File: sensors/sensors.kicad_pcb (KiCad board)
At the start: 2 copper layers, 73 x 56 mm, 73 parts, among them J1 GPIO, J3 JP_PWM, J4 JP_ADC, J5 JP_GPS, J6 JP_RADIO, J7 JP_RCIN, SW1 SW_SPDT_321, SW2 SW_SPDT_321, U1 SC16IS752IPW, U2 PCA9685PW, U3 ICM-42605, U4 IST8310, U5 MS5611-01BA, U6 74LVC1G86, U7 ADS1115IDGS, Y1 14.7456MHz, Y2 ASE-xxxMHz

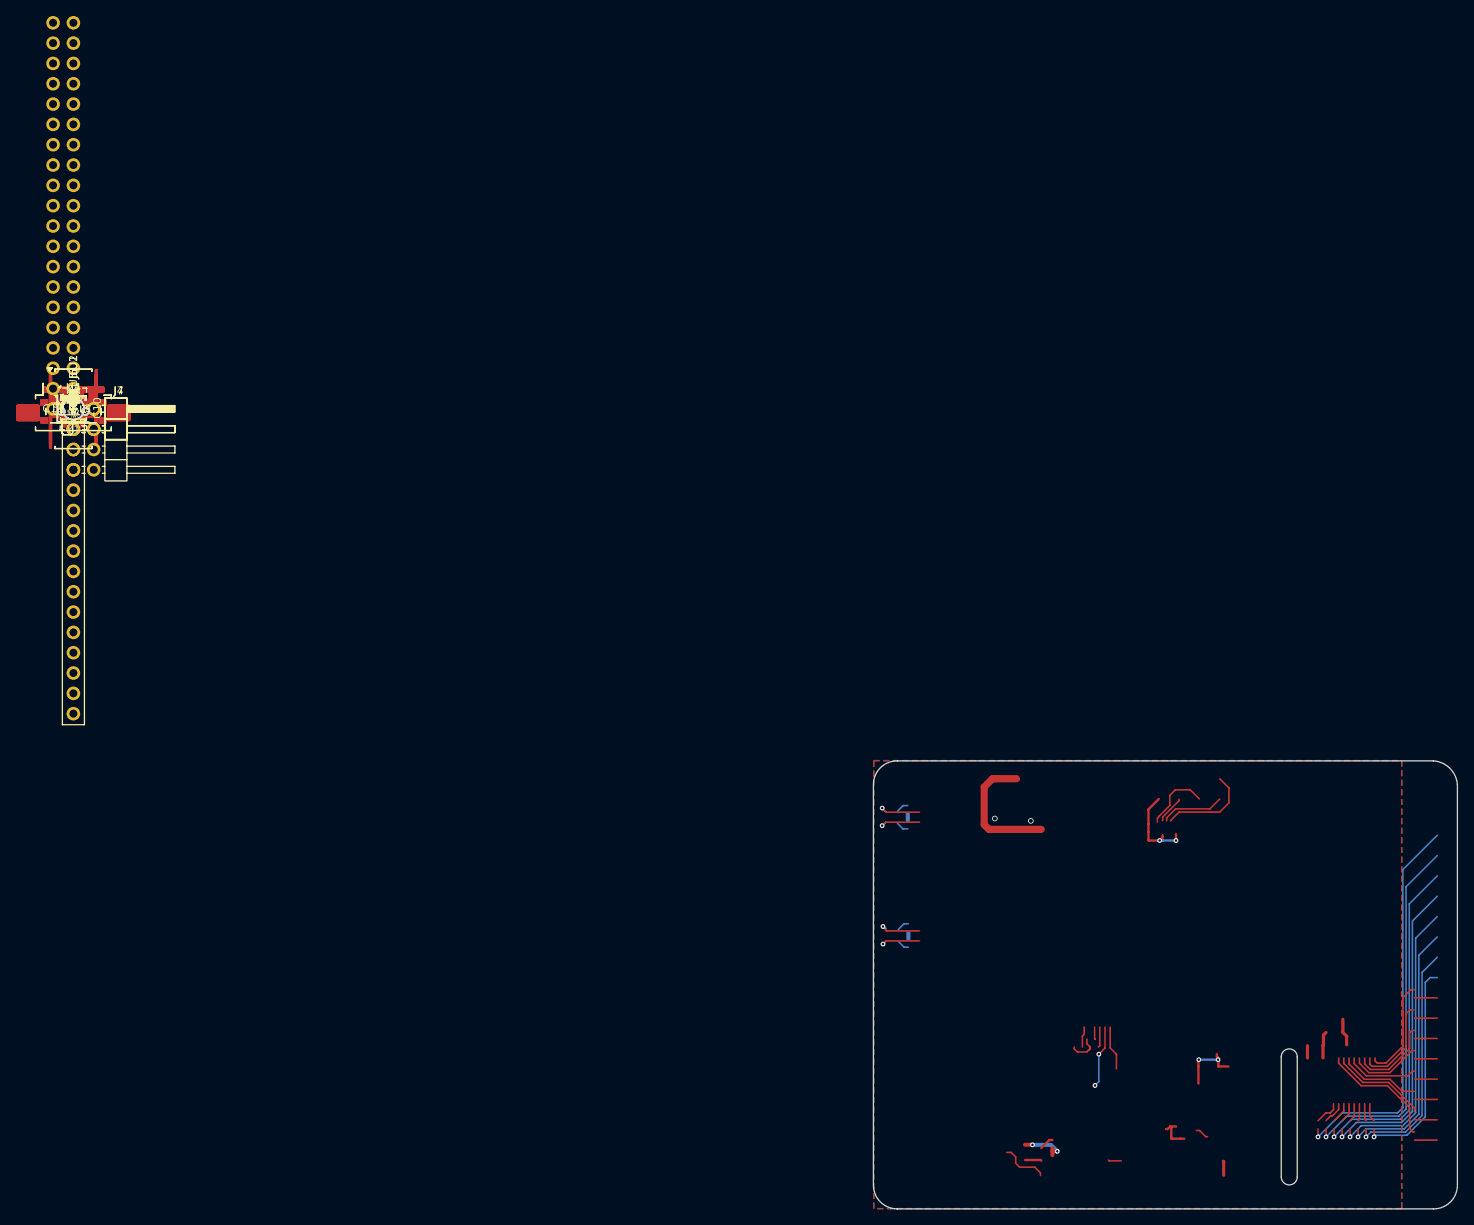
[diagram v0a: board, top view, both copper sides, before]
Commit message: routing
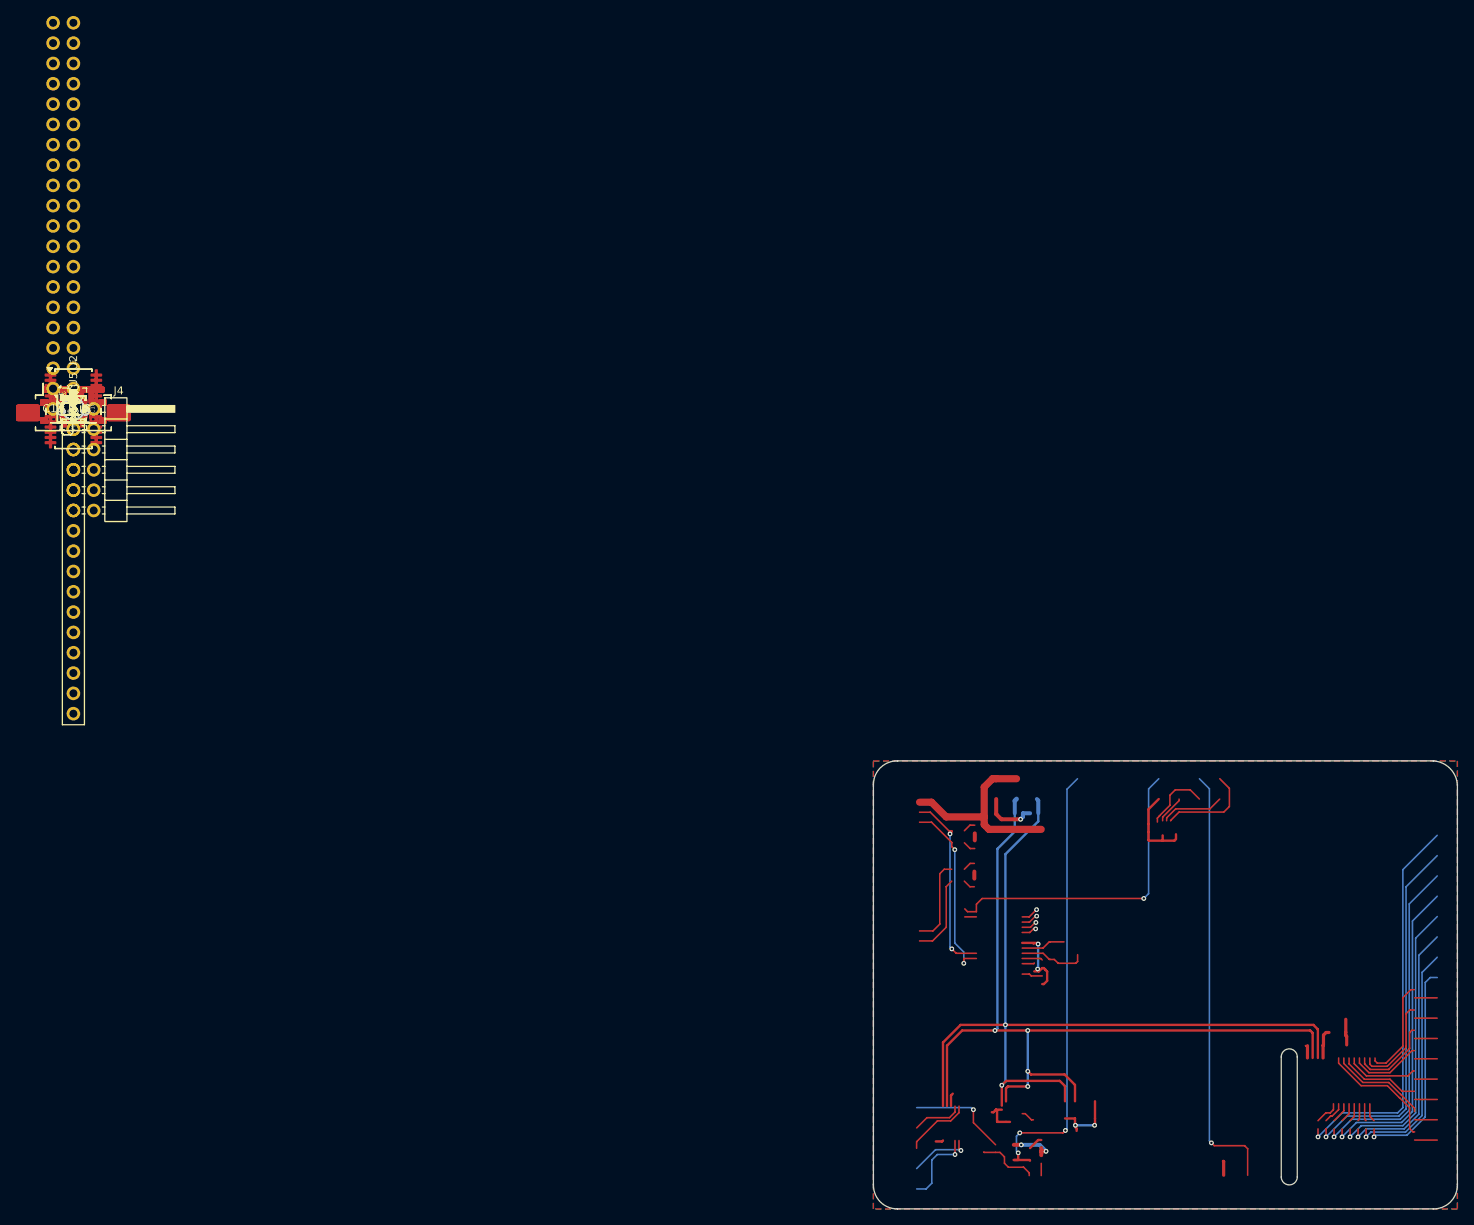
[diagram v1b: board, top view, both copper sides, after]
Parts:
- removed J7: JP_RCIN, Connector_PinHeader_2.54mm:PinHeader_2x02_P2.54mm_Horizontal
- D1: value RXA_GREEN -> TXA_RED; moved to F.Cu
- D2: value TXA_RED -> RXA_GREEN; moved to F.Cu
- D3: value RXB_GREEN -> TXB_RED; moved to F.Cu
- D4: value TXB_RED -> RXB_GREEN; moved to F.Cu
- J4: footprint Connector_PinHeader_2.54mm:PinHeader_2x04_P2.54mm_Horizontal -> Connector_PinHeader_2.54mm:PinHeader_2x06_P2.54mm_Horizontal
- R11, R6, R8, R9: moved to F.Cu
- R33, R34: moved to B.Cu
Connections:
- D1 pad 1: /UART/RXA -> /UART/TXA
- D2 pad 1: /UART/TXA -> /UART/RXA
- D3 pad 1: /UART/RXB -> /UART/TXB
- D4 pad 1: /UART/TXB -> /UART/RXB
- J4 pad 1: GND -> /ADC/AIN0
- J4 pad 3: GND -> /ADC/AIN1
- J4 pad 5: /ADC/AIN3 -> /ADC/AIN2
- J4 pad 6: /ADC/AIN2 -> GND
- J4 pad 7: /ADC/AIN1 -> /ADC/AIN3
- J4 pad 8: /ADC/AIN0 -> GND
- R10 pad 2: /UART/TXB -> /UART/RXB
- R7 pad 2: /UART/TXA -> /UART/RXA
- U6 pad 1: /RC inverter/RC -> /RCIN
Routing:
- net /GPIO3/SCL1: track 0.00 -> 110.1 mm, vias 0 -> 2
- net /GPIO2/SDA1: track 0.00 -> 107.7 mm, vias 0 -> 4
- net /GPIO15/RXD0: track 2.07 -> 56.7 mm, vias 0 -> 3
- net /GPIO25: track 0.00 -> 54.3 mm, vias 0 -> 1
- net /SDIODAT0/GPIO24: track 0.00 -> 39.5 mm, vias 0 -> 1
- net /UART/TXB: track 5.42 -> 23.2 mm, vias 1 -> 2
- net /UART/RXB: track 5.30 -> 23.0 mm, vias 1 -> 2
- net +3V3: track 39.4 -> 53.0 mm, vias 6 -> 7
- net /RCIN: track 0.00 -> 12.7 mm, vias 0 -> 1
- net /ADC/AIN0: track 0.00 -> 10.0 mm, vias 0 -> 1
- net +5V: track 18.1 -> 27.2 mm
- net /ADC/AIN2: track 0.00 -> 8.45 mm
- net /ADC/AIN1: track 0.00 -> 7.91 mm, vias 0 -> 1
- net /ADC/AIN3: track 0.00 -> 6.37 mm
- net /UART/TXA: track 5.40 -> 10.9 mm, vias 1 -> 0
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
